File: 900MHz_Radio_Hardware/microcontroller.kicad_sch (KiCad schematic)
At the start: 7 parts, among them U2 Teensy4.1_DEV-16771, U4 Opamp_Dual

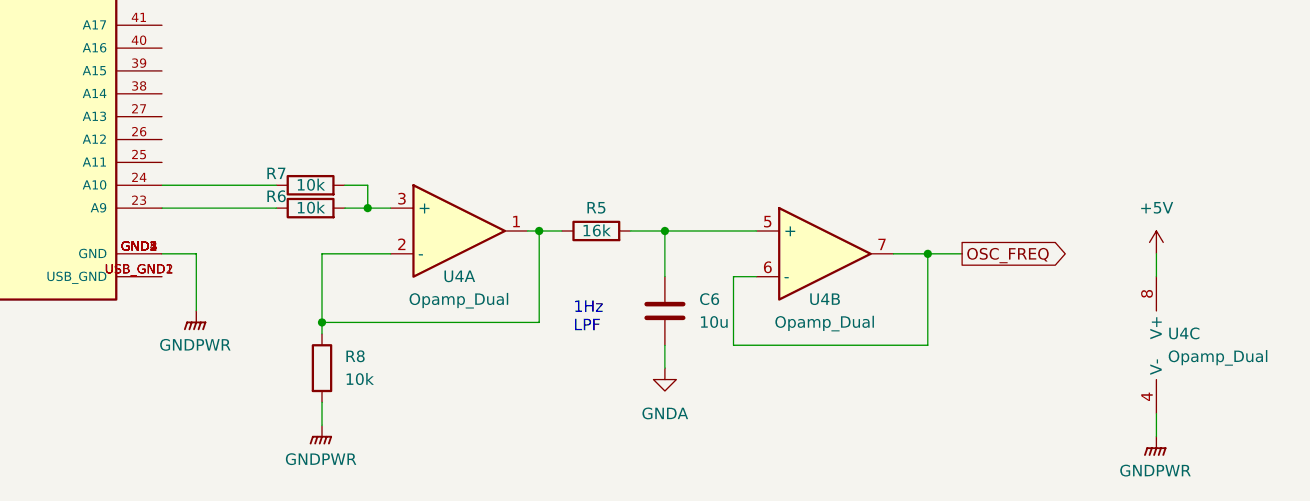
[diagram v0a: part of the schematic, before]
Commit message: Updated filter
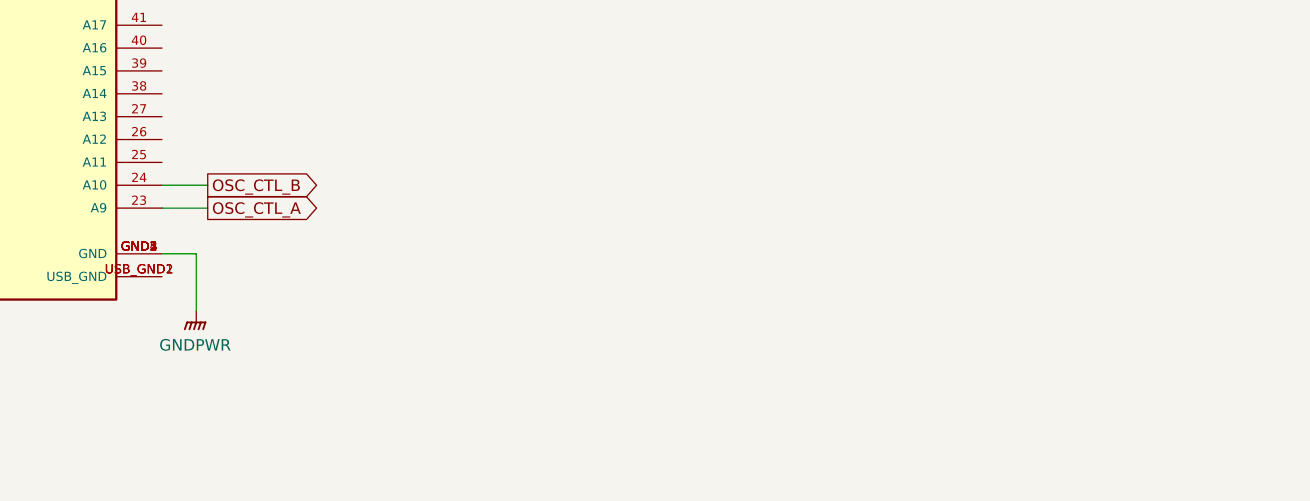
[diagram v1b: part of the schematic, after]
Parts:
- removed C6: 10u, symbol Device:C
- removed R5: 16k, symbol Device:R
- removed R6, R7, R8: 10k, symbol Device:R
- removed U4: Opamp_Dual, symbol Device:Opamp_Dual
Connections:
- net OSC_CTL_B: now reaches U2.24 (A10)
- net OSC_CTL_A: now reaches U2.23 (A9)
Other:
- note removed: "1Hz LPF"
